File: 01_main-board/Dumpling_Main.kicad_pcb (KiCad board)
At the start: 6 copper layers, 75 x 135.2 mm, 363 parts, among them J1 Conn_ARM_SWD_TagConnect_TC203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, J10 MICROMOD-2222-C, J11 USB_C_Receptacle_USB2.0_16P, J12 Conn_ARM_SWD_TagConnect_TC203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, J13 MICROMOD-2222-C, J14 USB_C_Receptacle_USB2.0_16P, J15 Conn_ARM_SWD_TagConnect_TC203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, J16 MICROMOD-2222-C, J17 USB_C_Receptacle_USB2.0_16P, J18 Conn_ARM_SWD_TagConnect_TC203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, J19 MICROMOD-2222-C, J2 Micro_SD_Card, J20 USB_C_Receptacle_USB2.0_16P, J21 Conn_ARM_SWD_TagConnect_TC203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, J22 MICROMOD-2222-C, J23 USB_C_Receptacle_USB2.0_16P, J3 USB_C_Receptacle_USB2.0_16P, J4 XT30PW-M, J5 SM04B-SRSS-TB, J6 Conn_ARM_SWD_TagConnect_TC203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, J7 MICROMOD-2222-C, J8 USB_C_Receptacle_USB2.0_16P, J9 Conn_ARM_SWD_TagConnect_TC203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, Q1 AO3401A, Q2 S8050, SW1 SW_DPST, SW10 SW_SPDT, SW11 SW_DPST, SW12 SW_SPDT, SW13 SW_DPST, SW14 SW_SPDT, SW2 SW_DPST, SW3 SW_DPST, SW4 SW_SPDT, SW5 SW_DPST, SW6 SW_SPDT, SW7 SW_DPST, SW8 SW_SPDT, SW9 SW_DPST, U1 STM32F405RGTx, U10 W25Q128JVS, U11 USBLC6-2SC6, U12 W25Q128JVS, U13 STM32F411CEUx, U14 USBLC6-2SC6, U15 W25Q128JVS, U16 STM32F411CEUx, U17 USBLC6-2SC6, U18 W25Q128JVS, U19 STM32F411CEUx, U2 USBLC6-2SC6, U20 USBLC6-2SC6, U22 STM32F411CEUx, U23 USBLC6-2SC6, U24 W25Q128JVS, U25 TPS562200, U26 TPS562200, U3 W25Q128JVS, U4 STM32F411CEUx, U5 STM32F411CEUx, U6 USBLC6-2SC6, U7 MPU-6050, U8 W25Q128JVS, U9 INA219AxDCN, Y1 32.768kHz, Y2 32.768kHz, Y3 32.768kHz, Y4 32.768kHz, Y5 32.768kHz, Y6 32.768kHz, Y7 32.768kHz

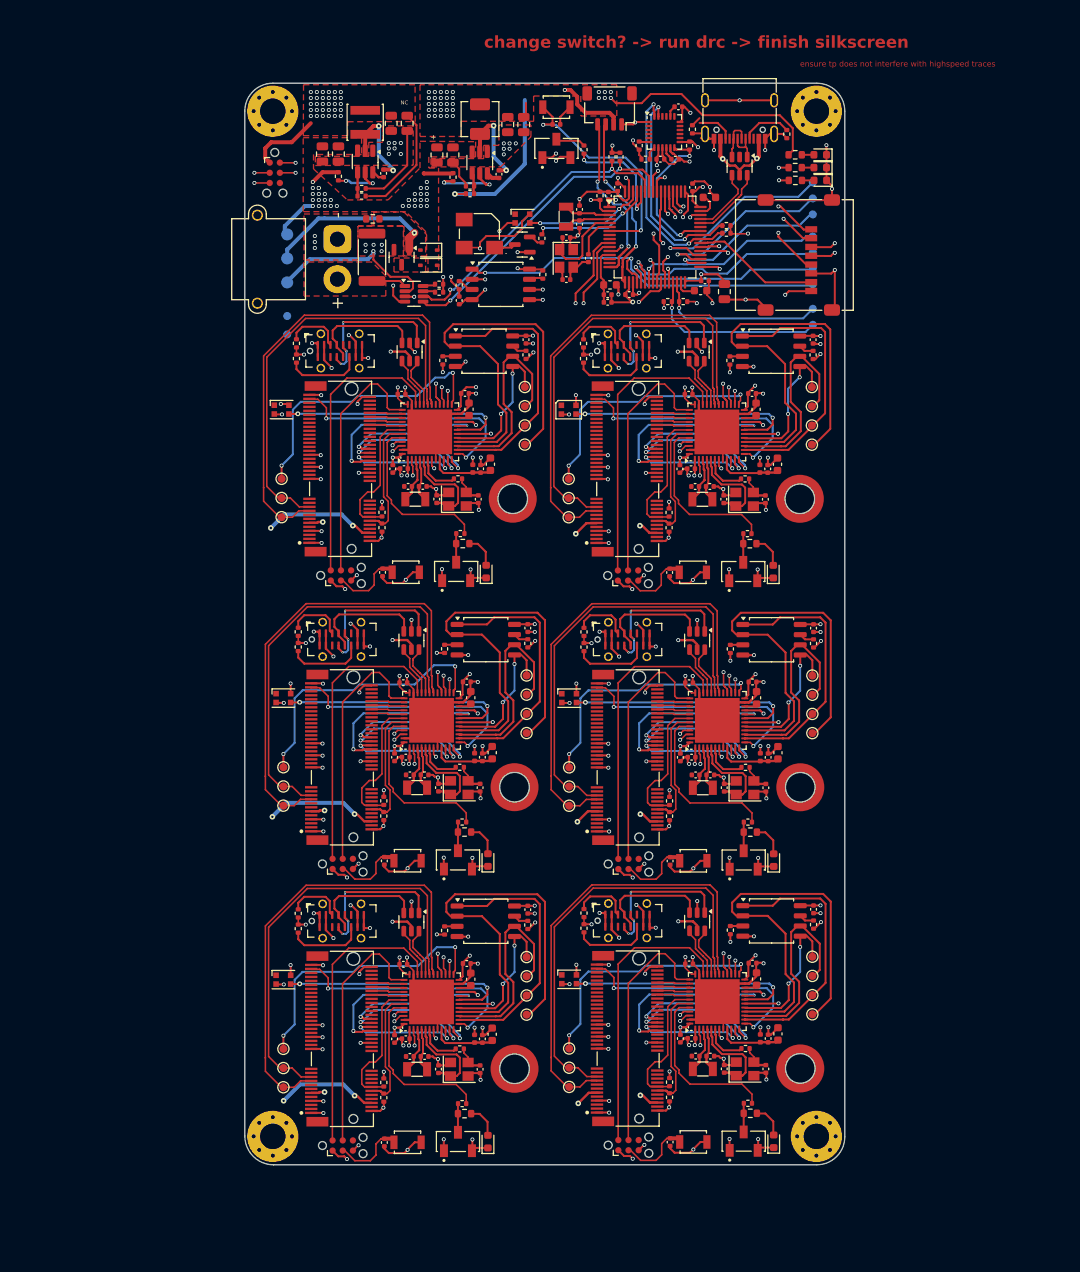
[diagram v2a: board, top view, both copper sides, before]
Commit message: ebay backboard
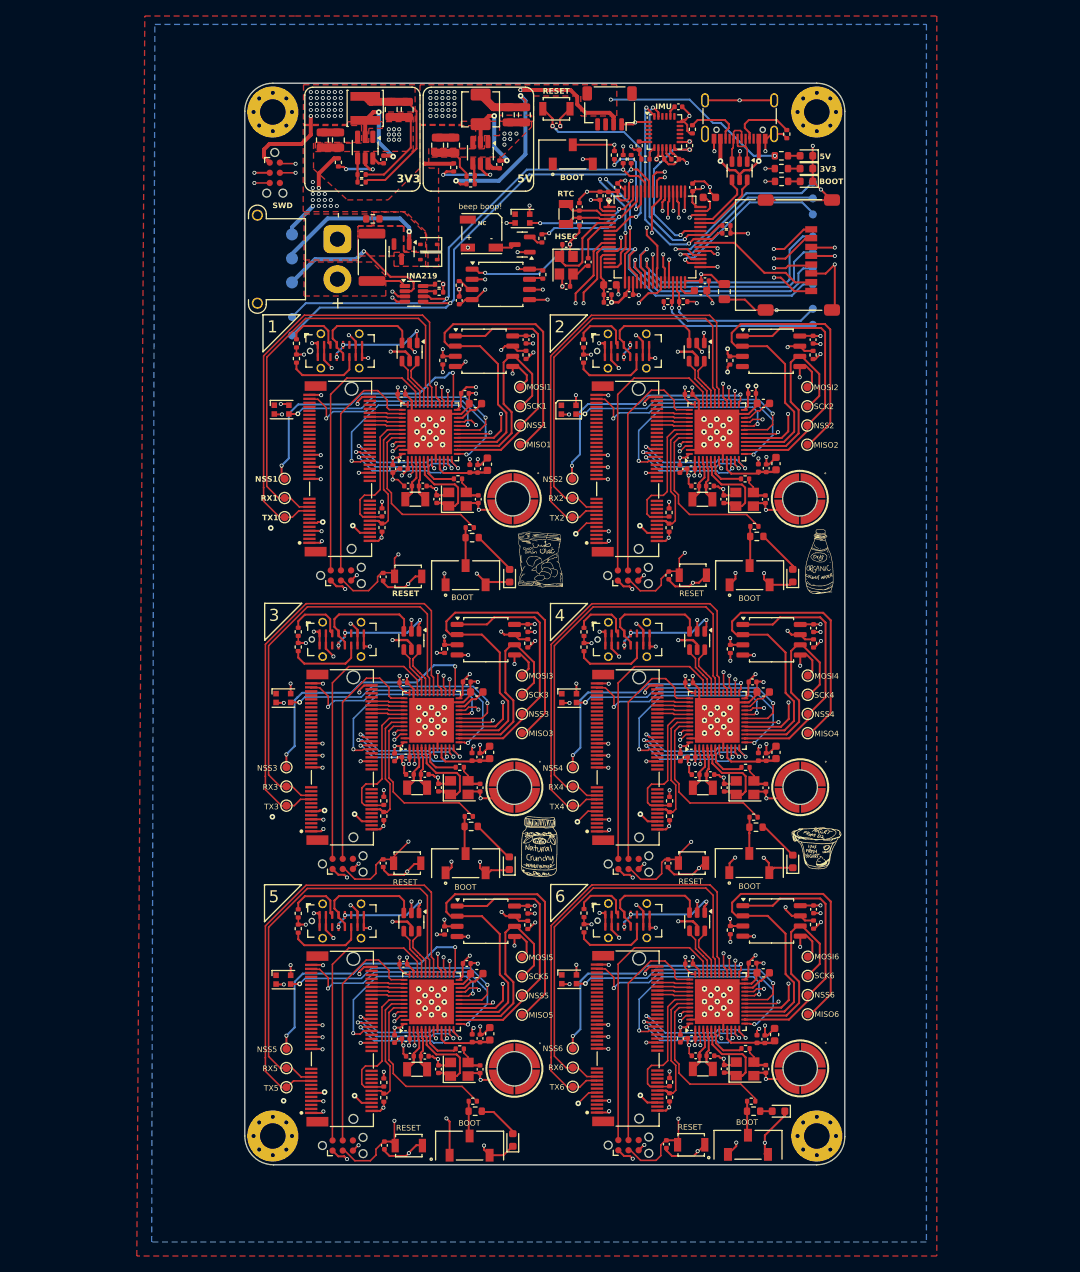
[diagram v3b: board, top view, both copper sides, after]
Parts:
- removed MP1, MP2, MP3, MP4, MP5, MP6: ~, WA-SMSI_9774XXX151:WA-SMSI_9774025151
- added G***: LOGO, LOGO, F.Cu at (205.2, 71.0)
- added G***: LOGO, LOGO, F.Cu at (165.0, 140.0)
- added G***: LOGO, LOGO, F.Cu at (165.4, 104.3)
- added G***: LOGO, LOGO, F.Cu at (130.3, 139.9)
- added G***: LOGO, LOGO, F.Cu at (130.4, 104.0)
- added G***: LOGO, LOGO, B.Cu at (132.7, 59.3)
- added G***: LOGO, LOGO, B.Cu at (132.4, 73.2)
- added U21: SMTSOM2_525STR, SMTSOM2.525STR:SMD_BD5.6-D4.1, F.Cu at (162.9, 132.4)
- added U27: SMTSOM2_525STR, SMTSOM2.525STR:SMD_BD5.6-D4.1, F.Cu at (127.2, 132.4)
- added U28: SMTSOM2_525STR, SMTSOM2.525STR:SMD_BD5.6-D4.1, F.Cu at (127.0, 96.3)
- added U29: SMTSOM2_525STR, SMTSOM2.525STR:SMD_BD5.6-D4.1, F.Cu at (162.9, 167.6)
- added U30: SMTSOM2_525STR, SMTSOM2.525STR:SMD_BD5.6-D4.1, F.Cu at (127.2, 167.6)
- added U31: SMTSOM2_525STR, SMTSOM2.525STR:SMD_BD5.6-D4.1, F.Cu at (162.9, 96.4)
- BZ1: footprint CSS-0575B-SMT:CUI_CSS-0575B-SMT -> FST-5030:BUZ-SMD_FST-5030
- SW1: value SW_DPST -> SW_SPDT; footprint CJS-1200TA:SW_CJS-1200TA -> JS102011JCQN:SW_JS102011JCQN
- SW10, SW12, SW14, SW4, SW6, SW8: footprint CJS-1200TA:SW_CJS-1200TA -> JS102011JCQN:SW_JS102011JCQN
- SW11, SW13, SW2, SW3, SW5, SW7, SW9: value SW_DPST -> SW_SPST
- moved R2 3.86 mm to (139.7, 53.4)
- moved D17 3.81 mm to (160.2, 172.9), turned to 180 degrees
- moved D15 3.11 mm to (127.0, 176.5)
- moved D4 2.98 mm to (126.6, 106.0)
- moved D11 2.69 mm to (126.6, 141.9)
- moved D9 2.49 mm to (162.0, 106.0)
- moved D13 2.39 mm to (162.0, 141.7)
- moved SW1 2.18 mm to (134.5, 53.3)
- moved C34 1.74 mm to (111.8, 47.7)
- moved C38 1.74 mm to (113.8, 47.7)
- moved L2 1.74 mm to (108.5, 47.5)
- moved R16 1.74 mm to (108.1, 56.8)
- moved C31 1.74 mm to (103.2, 51.5)
- moved C32 1.74 mm to (105.2, 51.5)
- moved C33 1.74 mm to (110.8, 53.9)
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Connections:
- J11 pad B8: unconnected-(J11-SBU1-PadA8) -> unconnected-(J11-SBU2-PadB8)
- J14 pad B8: unconnected-(J14-SBU1-PadA8) -> unconnected-(J14-SBU2-PadB8)
- J17 pad B8: unconnected-(J17-SBU1-PadA8) -> unconnected-(J17-SBU2-PadB8)
- J20 pad B8: unconnected-(J20-SBU1-PadA8) -> unconnected-(J20-SBU2-PadB8)
- J23 pad B8: unconnected-(J23-SBU1-PadA8) -> unconnected-(J23-SBU2-PadB8)
- J8 pad B8: unconnected-(J8-SBU1-PadA8) -> unconnected-(J8-SBU2-PadB8)
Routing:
- net GND: track 465.1 -> 644.8 mm, vias 178 -> 257
- net NRST: track 29.6 -> 69.4 mm
- net co6_FLASH_HOLD: track 3.30 -> 41.2 mm, vias 1 -> 2
- net co4_FLASH_HOLD: track 3.30 -> 39.8 mm, vias 1 -> 2
- net co2_FLASH_HOLD: track 3.30 -> 38.6 mm, vias 1 -> 2
- net co2_FLASH_WP: track 3.62 -> 32.6 mm, vias 1 -> 2
- net co6_FLASH_WP: track 3.62 -> 31.5 mm, vias 1 -> 2
- net co4_FLASH_WP: track 3.62 -> 31.4 mm, vias 1 -> 2
- net co1_FLASH_HOLD: track 3.30 -> 28.3 mm, vias 1 -> 2
- net co5_FLASH_HOLD: track 3.30 -> 28.2 mm, vias 1 -> 2
- net co3_FLASH_HOLD: track 3.30 -> 28.1 mm, vias 1 -> 2
- net I2C1_SCL: track 38.8 -> 62.9 mm
- net Net-(SW1-B): track 4.95 -> 28.1 mm, vias 1 -> 2
- net I2C1_SDA: track 38.0 -> 60.9 mm
- net co1_FLASH_WP: track 3.62 -> 23.5 mm, vias 1 -> 2
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- added copper zone on B.Cu, net GND
- added copper zone on In3.Cu, net GND
- added copper zone on In4.Cu, net GND
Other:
- board text added: "1"
- board text added: "2"
- board text added: "3"
- board text added: "3V3"
- board text added: "4"
- board text added: "5"
- board text added: "5V"
- board text added: "6"
- board text added: "BOOT"
- board text added: "Data Dumpling Payload v0.1 04/25 @seoyoonij"
- board text added: "F411"
- board text added: "FLASH"
- board text added: "HSEC"
- board text added: "IMU"
- board text added: "INA219"
- board text added: "MISO1"
- board text added: "MISO2"
- board text added: "MISO3"
- board text added: "MISO4"
- board text added: "MISO5"
- board text added: "MISO6"
- board text added: "MOSI1"
- board text added: "MOSI2"
- board text added: "MOSI3"
- board text added: "MOSI4"
- board text added: "MOSI5"
- board text added: "MOSI6"
- board text added: "NSS1"
- board text added: "NSS2"
- board text added: "NSS3"
- board text added: "NSS4"
- board text added: "NSS5"
- board text added: "NSS6"
- board text added: "RESET"
- board text added: "RTC"
- board text added: "RX"
- board text added: "RX1"
- board text added: "RX2"
- board text added: "RX3"
- board text added: "RX4"
- board text added: "RX5"
- board text added: "RX6"
- board text added: "SCK1"
- board text added: "SCK2"
- board text added: "SCK3"
- board text added: "SCK4"
- board text added: "SCK5"
- board text added: "SCK6"
- board text added: "SCL1"
- board text added: "SCL2"
- board text added: "SDA1"
- board text added: "SDA2"
- board text added: "SWD"
- board text added: "TX"
- board text added: "TX1"
- board text added: "TX2"
- board text added: "TX3"
- board text added: "TX4"
- board text added: "TX5"
- board text added: "TX6"
- board text added: "VBAT"
- board text added: "VBUS"
- board text added: "VIN"
- board text added: "beep boop!"
- board text added: "let's not fuck up the board!"
- board text removed: "change switch? -> run drc -> finish silkscreen"
- board text removed: "ensure tp does not interfere with highspeed traces"
